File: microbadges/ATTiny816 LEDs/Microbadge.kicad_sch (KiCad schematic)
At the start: 13 parts, among them U1 ATtiny816-M

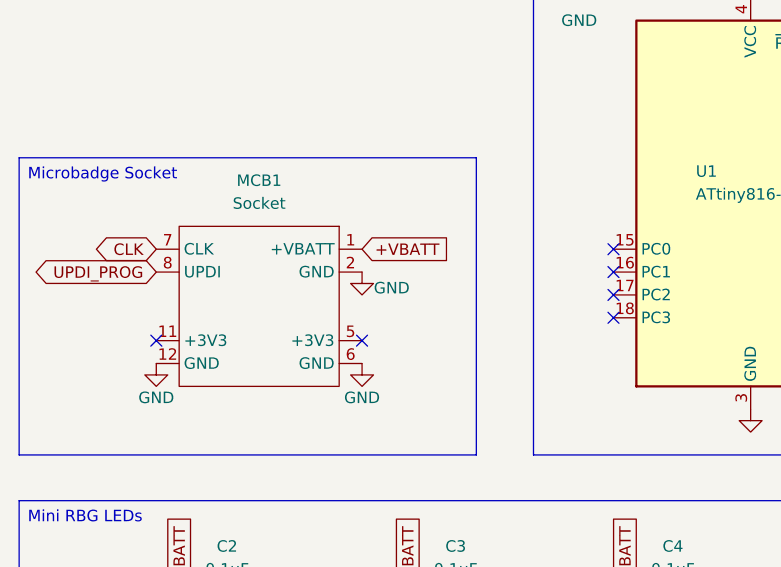
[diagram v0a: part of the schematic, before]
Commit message: Update to Bit-banged I2C
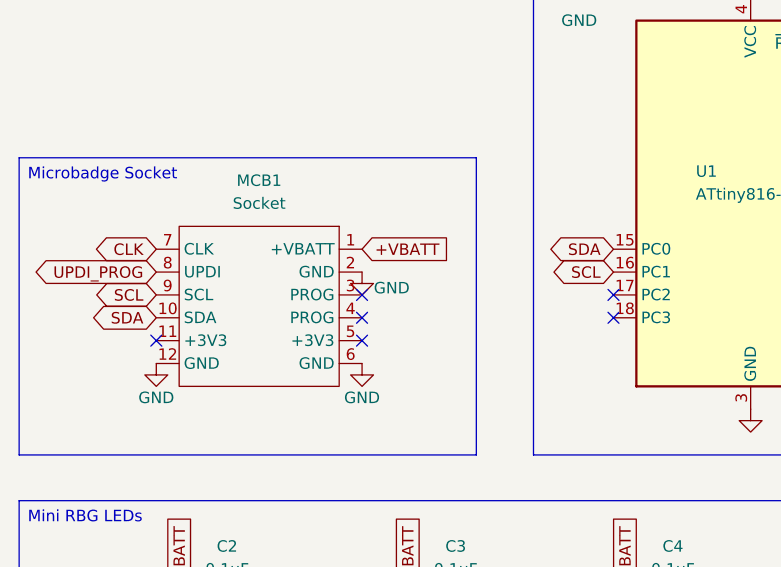
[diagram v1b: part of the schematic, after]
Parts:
- MCB1: footprint Microbadge V2:Microbadge_V2_simple_round -> Microbadge V2:Microbadge_V2_full_round; symbol Microbadge V2:Microbadge_V2_simple -> Microbadge V2:Microbadge_V2_full; now in the parts list
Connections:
- net SDA: now reaches U1.15 (PC0)
- net SDA: now also MCB1.10 (SDA)
- net SCL: now reaches U1.16 (PC1)
- net SCL: now also MCB1.9 (SCL)
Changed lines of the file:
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@@
+	)
+	(no_connect
+		(at 124.46 82.55)
+	)
+	(no_connect
+		(at 124.46 85.09)
 	)
 	(no_connect
@@
 	)
 	(no_connect
-		(at 152.4 80.01)
-	)
-	(no_connect
 		(at 182.88 69.85)
 	)
@@
 	(no_connect
 		(at 195.58 128.27)
-	)
-	(no_connect
-		(at 152.4 77.47)
 	)
 	(no_connect
@@
 		)
 	)
+	(global_label "SDA"
+		(shape bidirectional)
+		(at 152.4 77.47 180)
+		(fields_autoplaced yes)
+		(effects
+			(font
+				(size 1.27 1.27)
+			)
+			(justify right)
+		)
+		(property "Intersheetrefs" "${INTERSHEET_REFS}"
+			(at 144.7354 77.47 0)
+			(effects
+				(font
+					(size 1.27 1.27)
+				)
+				(justify right)
+				(hide yes)
+			)
+		)
+	)
 	(global_label "+VBATT"
 		(shape input)
@@
 		)
 	)
+	(global_label "SDA"
+		(shape bidirectional)
+		(at 101.6 85.09 180)
+		(fields_autoplaced yes)
+		(effects
+			(font
+				(size 1.27 1.27)
+			)
+			(justify right)
+		)
+		(property "Intersheetrefs" "${INTERSHEET_REFS}"
+			(at 93.9354 85.09 0)
+			(effects
+				(font
+					(size 1.27 1.27)
+				)
+				(justify right)
+				(hide yes)
+			)
+		)
+	)
 	(global_label "UPDI_PROG"
 		(shape bidirectional)
@@
 		)
 	)
+	(global_label "SCL"
+		(shape bidirectional)
+		(at 152.4 80.01 180)
+		(fields_autoplaced yes)
+		(effects
+			(font
+				(size 1.27 1.27)
+			)
+			(justify right)
+		)
+		(property "Intersheetrefs" "${INTERSHEET_REFS}"
+			(at 144.7959 80.01 0)
+			(effects
+				(font
+					(size 1.27 1.27)
+				)
+				(justify right)
+				(hide yes)
+			)
+		)
+	)
 	(global_label "+VBATT"
 		(shape input)
@@
 				)
 				(justify left)
+				(hide yes)
+			)
+		)
+	)
+	(global_label "SCL"
+		(shape bidirectional)
+		(at 101.6 82.55 180)
+		(fields_autoplaced yes)
+		(effects
+			(font
+				(size 1.27 1.27)
+			)
+			(justify right)
+		)
+		(property "Intersheetrefs" "${INTERSHEET_REFS}"
+			(at 93.9959 82.55 0)
+			(effects
+				(font
+					(size 1.27 1.27)
+				)
+				(justify right)
 				(hide yes)
 			)
@@
 	)
 	(symbol
-		(lib_id "Microbadge V2:Microbadge_V2_simple")
+		(lib_id "Microbadge V2:Microbadge_V2_full")
 		(at 113.03 83.82 270)
 		(unit 1)
 		(exclude_from_sim no)
-		(in_bom no)
+		(in_bom yes)
 		(on_board yes)
 		(dnp no)
@@
 			)
 		)
-		(property "Footprint" "Microbadge V2:Microbadge_V2_simple_round"
+		(property "Footprint" "Microbadge V2:Microbadge_V2_full_round"
 			(at 113.03 83.82 0)
 			(effects
@@
 		(pin "2"
 		)
+		(pin "10"
+		)
+		(pin "9"
+		)
+		(pin "3"
+		)
+		(pin "4"
+		)
 		(instances
